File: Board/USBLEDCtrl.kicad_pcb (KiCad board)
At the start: 2 copper layers, 40 x 50 mm, 23 parts, among them IC1 ATTINY861A-S, P1 CONN_PWR, P2 CONN_ISP, P3 CONN_USB, P4 CONN_LED, Q1 Q_NMOS_GDS, Q2 Q_NMOS_GDS, Q3 Q_NMOS_GDS, U1 LT1129CST-3.3, Y1 12MHz

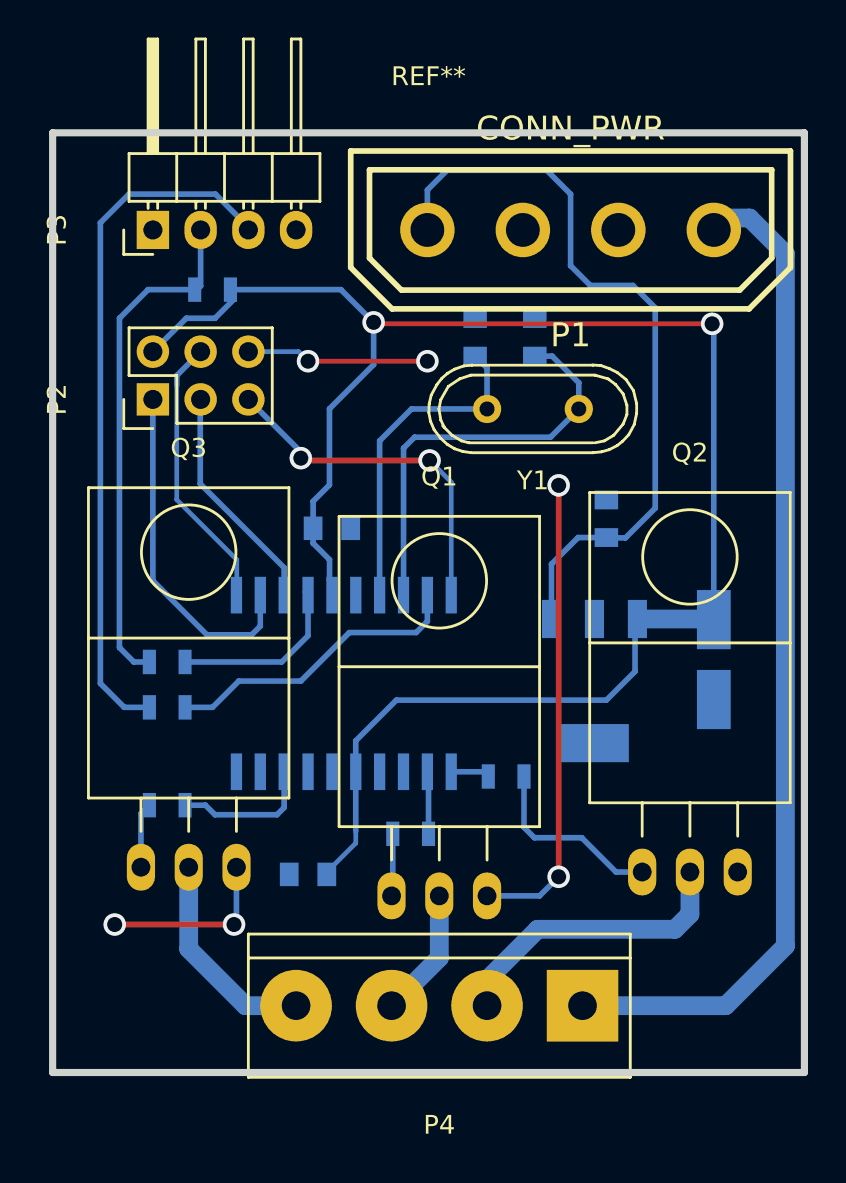
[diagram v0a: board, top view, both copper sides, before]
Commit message: Grössere Restringe
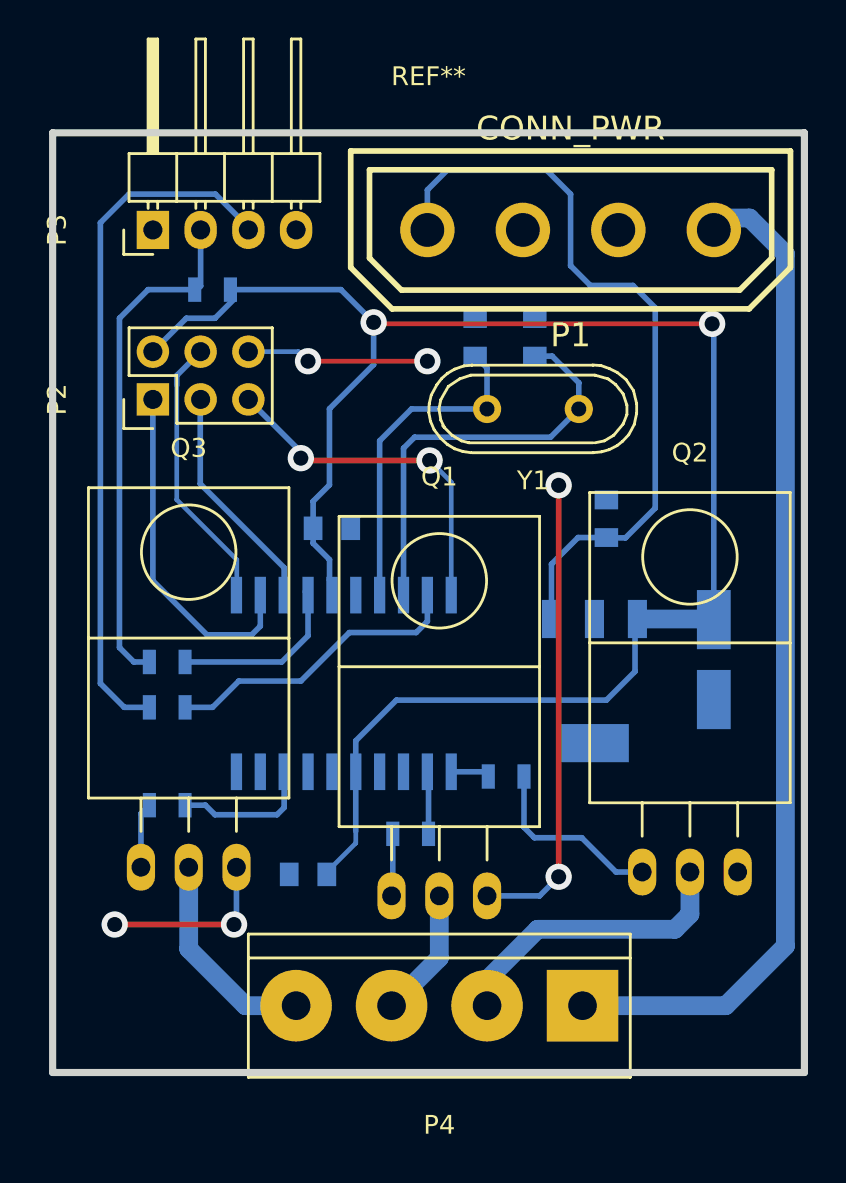
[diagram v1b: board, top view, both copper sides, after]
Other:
- net class Default: via_dia 1.2 -> 1.4
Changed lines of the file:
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@@
     (segment_width 0.2)
     (edge_width 0.15)
-    (via_size 1.2)
+    (via_size 1.4)
     (via_drill 0.8)
     (via_min_size 0.4)
@@
     (clearance 0.2)
     (trace_width 0.25)
-    (via_dia 1.2)
+    (via_dia 1.4)
     (via_drill 0.8)
     (uvia_dia 0.3)
@@
     (fp_line (start 0 -49.9999) (end 0 0) (layer Edge.Cuts) (width 0.381))
   )
-  (segment (start 125.73 74.422) (end 128.397 74.422) (width 0.25) (layer B.Cu) (net 1) (status 400000))
-  (via (at 135.255 74.93) (size 1.2) (drill 0.8) (layers F.Cu B.Cu) (net 1))
+  (segment (start 125.73 74.422) (end 128.397 74.422) (width 0.25) (layer B.Cu) (net 1))
+  (via (at 135.255 74.93) (size 1.4) (drill 0.8) (layers F.Cu B.Cu) (net 1))
   (segment (start 128.905 74.93) (end 135.255 74.93) (width 0.25) (layer F.Cu) (net 1))
-  (via (at 128.905 74.93) (size 1.2) (drill 0.8) (layers F.Cu B.Cu) (net 1))
+  (via (at 128.905 74.93) (size 1.4) (drill 0.8) (layers F.Cu B.Cu) (net 1))
   (segment (start 128.397 74.422) (end 128.905 74.93) (width 0.25) (layer B.Cu) (net 1))
   (segment (start 124.968 104.902) (end 118.618 104.902) (width 0.3) (layer F.Cu) (net 1))
-  (via (at 118.618 104.902) (size 1.2) (drill 0.8) (layers F.Cu B.Cu) (net 1))
+  (via (at 118.618 104.902) (size 1.4) (drill 0.8) (layers F.Cu B.Cu) (net 1))
   (segment (start 125.095 101.854) (end 125.095 104.775) (width 0.3) (layer B.Cu) (net 1) (status 10))
   (segment (start 125.095 104.775) (end 124.968 104.902) (width 0.3) (layer B.Cu) (net 1))
-  (via (at 124.968 104.902) (size 1.2) (drill 0.8) (layers F.Cu B.Cu) (net 1))
+  (via (at 124.968 104.902) (size 1.4) (drill 0.8) (layers F.Cu B.Cu) (net 1))
   (segment (start 142.24 102.362) (end 142.24 81.534) (width 0.3) (layer F.Cu) (net 1))
-  (via (at 142.24 81.534) (size 1.2) (drill 0.8) (layers F.Cu B.Cu) (net 1))
+  (via (at 142.24 81.534) (size 1.4) (drill 0.8) (layers F.Cu B.Cu) (net 1))
   (segment (start 138.43 103.378) (end 141.224 103.378) (width 0.3) (layer B.Cu) (net 1) (status 10))
   (segment (start 141.224 103.378) (end 142.24 102.362) (width 0.3) (layer B.Cu) (net 1))
-  (via (at 142.24 102.362) (size 1.2) (drill 0.8) (layers F.Cu B.Cu) (net 1))
+  (via (at 142.24 102.362) (size 1.4) (drill 0.8) (layers F.Cu B.Cu) (net 1))
   (segment (start 132.715 87.375) (end 132.715 79.163801) (width 0.3) (layer B.Cu) (net 2) (status 10))
   (segment (start 132.715 79.163801) (end 134.408801 77.47) (width 0.3) (layer B.Cu) (net 2))
@@
   (segment (start 150.406586 72.939555) (end 132.472731 72.939555) (width 0.25) (layer F.Cu) (net 13))
   (segment (start 132.472731 72.939555) (end 132.395033 72.861857) (width 0.25) (layer F.Cu) (net 13))
-  (via (at 132.395033 72.861857) (size 1.2) (drill 0.8) (layers F.Cu B.Cu) (net 13))
+  (via (at 132.395033 72.861857) (size 1.4) (drill 0.8) (layers F.Cu B.Cu) (net 13))
   (segment (start 150.495 73.027969) (end 150.406586 72.939555) (width 0.3) (layer B.Cu) (net 13))
   (segment (start 150.495 88.67902) (end 150.495 73.027969) (width 0.3) (layer B.Cu) (net 13) (status 10))
-  (via (at 150.406586 72.939555) (size 1.2) (drill 0.8) (layers F.Cu B.Cu) (net 13))
+  (via (at 150.406586 72.939555) (size 1.4) (drill 0.8) (layers F.Cu B.Cu) (net 13))
   (segment (start 133.604 92.964) (end 131.445 95.123) (width 0.3) (layer B.Cu) (net 13))
   (segment (start 131.445 95.123) (end 131.445 96.775) (width 0.3) (layer B.Cu) (net 13) (status 20))
@@
   (segment (start 128.642847 80.210082) (end 128.520797 80.088032) (width 0.3) (layer F.Cu) (net 17))
   (segment (start 135.37313 80.210082) (end 128.642847 80.210082) (width 0.3) (layer F.Cu) (net 17))
-  (via (at 128.520797 80.088032) (size 1.2) (drill 0.8) (layers F.Cu B.Cu) (net 17))
+  (via (at 128.520797 80.088032) (size 1.4) (drill 0.8) (layers F.Cu B.Cu) (net 17))
   (segment (start 135.121374 79.958326) (end 135.37313 80.210082) (width 0.25) (layer F.Cu) (net 17))
   (segment (start 136.525 81.361952) (end 135.37313 80.210082) (width 0.25) (layer B.Cu) (net 17))
   (segment (start 136.525 87.375) (end 136.525 81.361952) (width 0.25) (layer B.Cu) (net 17) (status 10))
-  (via (at 135.37313 80.210082) (size 1.2) (drill 0.8) (layers F.Cu B.Cu) (net 17))
+  (via (at 135.37313 80.210082) (size 1.4) (drill 0.8) (layers F.Cu B.Cu) (net 17))
   (segment (start 150.495 67.31) (end 152.4 67.31) (width 1) (layer B.Cu) (net 18) (status 10))
   (segment (start 152.4 67.31) (end 154.305 69.215) (width 1) (layer B.Cu) (net 18))

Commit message: Layout done
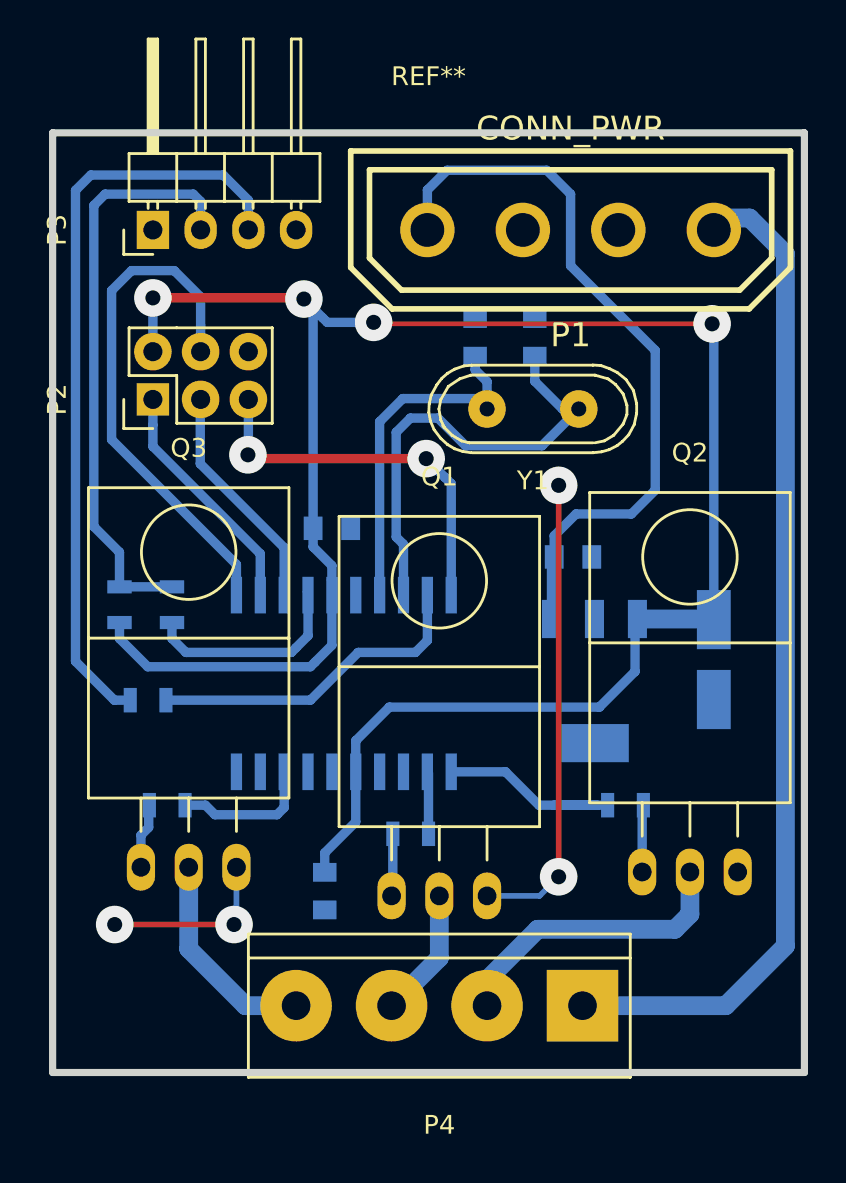
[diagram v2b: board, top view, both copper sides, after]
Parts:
- moved R6 17.5 mm to (118.9, 87.9), turned to 270 degrees
- moved R1 6.53 mm to (145.8, 98.6)
- moved R4 3.06 mm to (121.7, 87.9), turned to 270 degrees
- moved C1 2.70 mm to (143.0, 85.3), turned to 0 degrees
- moved C3 1.26 mm to (129.8, 103.1), turned to 270 degrees
- moved R5 1.09 mm to (120.4, 93.0)
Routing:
- net +3V3: track 95.4 -> 112.2 mm, vias 2 -> 4
- net Net-(IC1-Pad1): track 14.8 -> 27.6 mm
- net GND: track 44.2 -> 34.5 mm, vias 6 -> 4
- net Net-(IC1-Pad11): track 2.17 -> 11.4 mm
- net Net-(Q2-Pad1): track 9.98 -> 3.58 mm
- net Net-(IC1-Pad2): track 17.9 -> 12.9 mm
- net Net-(P3-Pad2): track 27.9 -> 32.3 mm
- net Net-(P3-Pad3): track 37.0 -> 40.8 mm
- net Net-(C6-Pad2): track 22.3 -> 24.6 mm
- net Net-(IC1-Pad4): track 10.2 -> 11.8 mm
- net Net-(IC1-Pad9): track 16.9 -> 18.3 mm
- net Net-(IC1-Pad10): track 19.2 -> 20.4 mm
- net +5V: track 40.3 -> 39.2 mm
- net Net-(C5-Pad2): track 17.7 -> 18.8 mm
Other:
- net class Default: via_dia 1.4 -> 2
